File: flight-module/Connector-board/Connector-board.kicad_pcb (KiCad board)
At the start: 4 copper layers, 141.7 x 134.1 mm, 39 parts, among them J1 DB9_Female, J2 Stack_Shape, J3 DB9_Female, J4 DB15_Female, J5 DB25_Receptacle, U1 MAX31855KASA, U2 MAX31855KASA, U3 MAX31855KASA, U4 MAX31855KASA

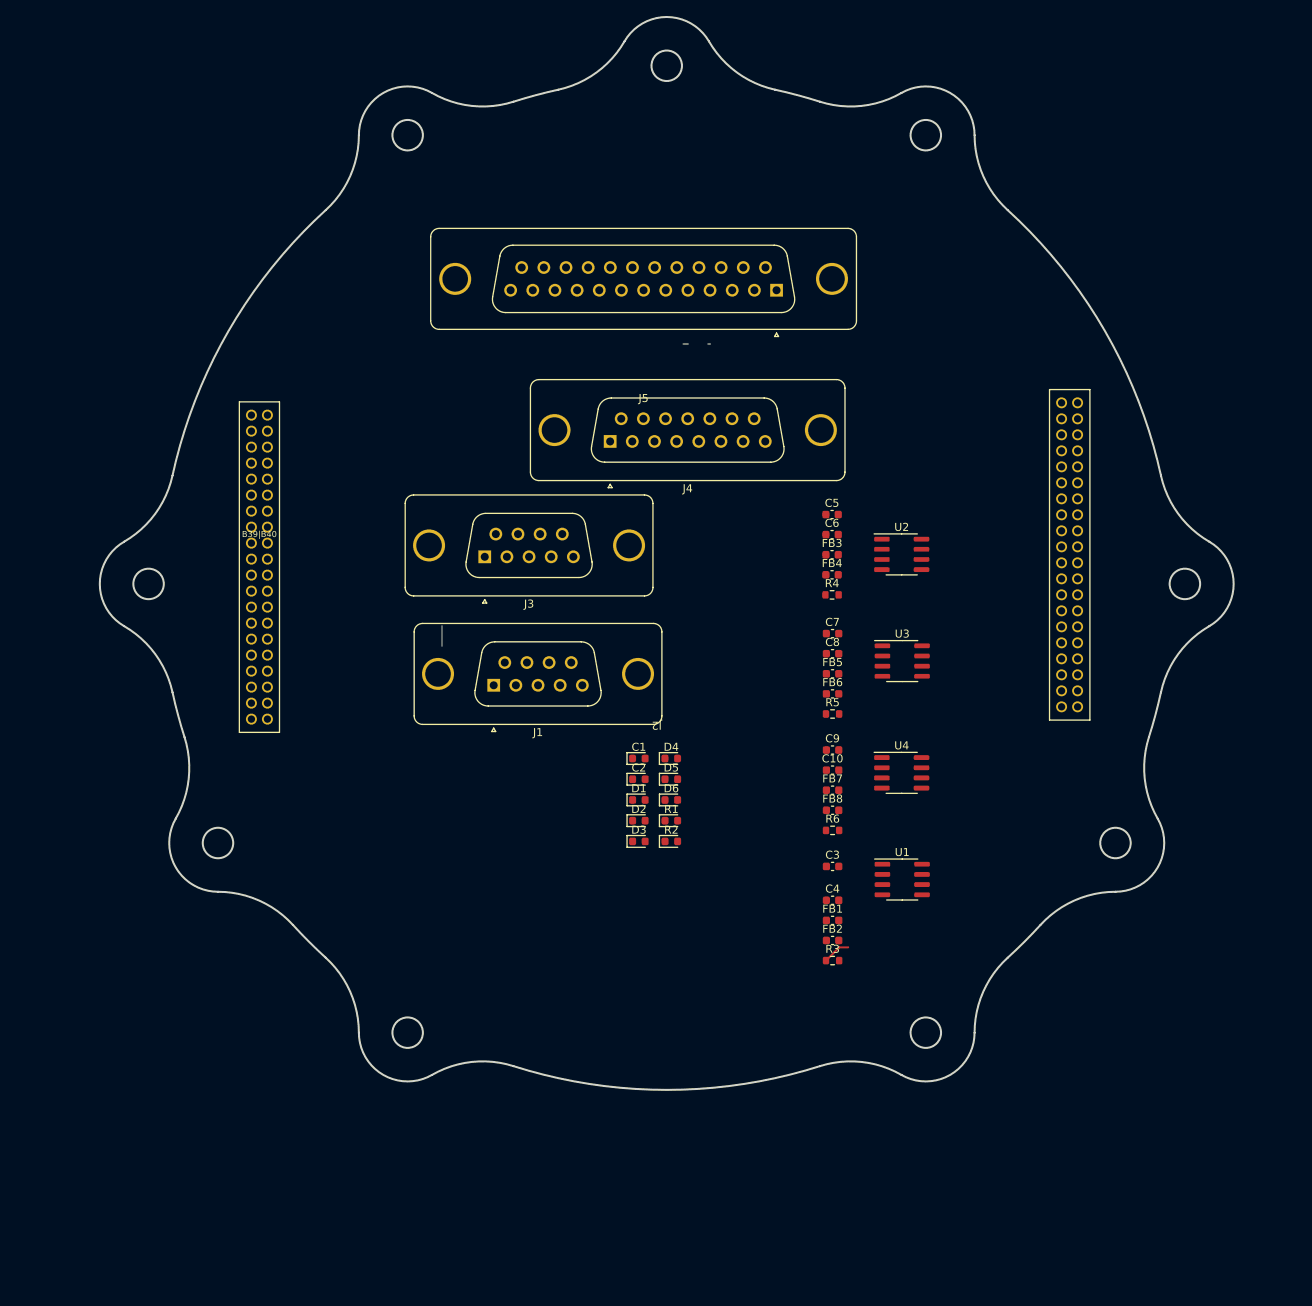
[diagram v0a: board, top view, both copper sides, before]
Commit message: completed routing
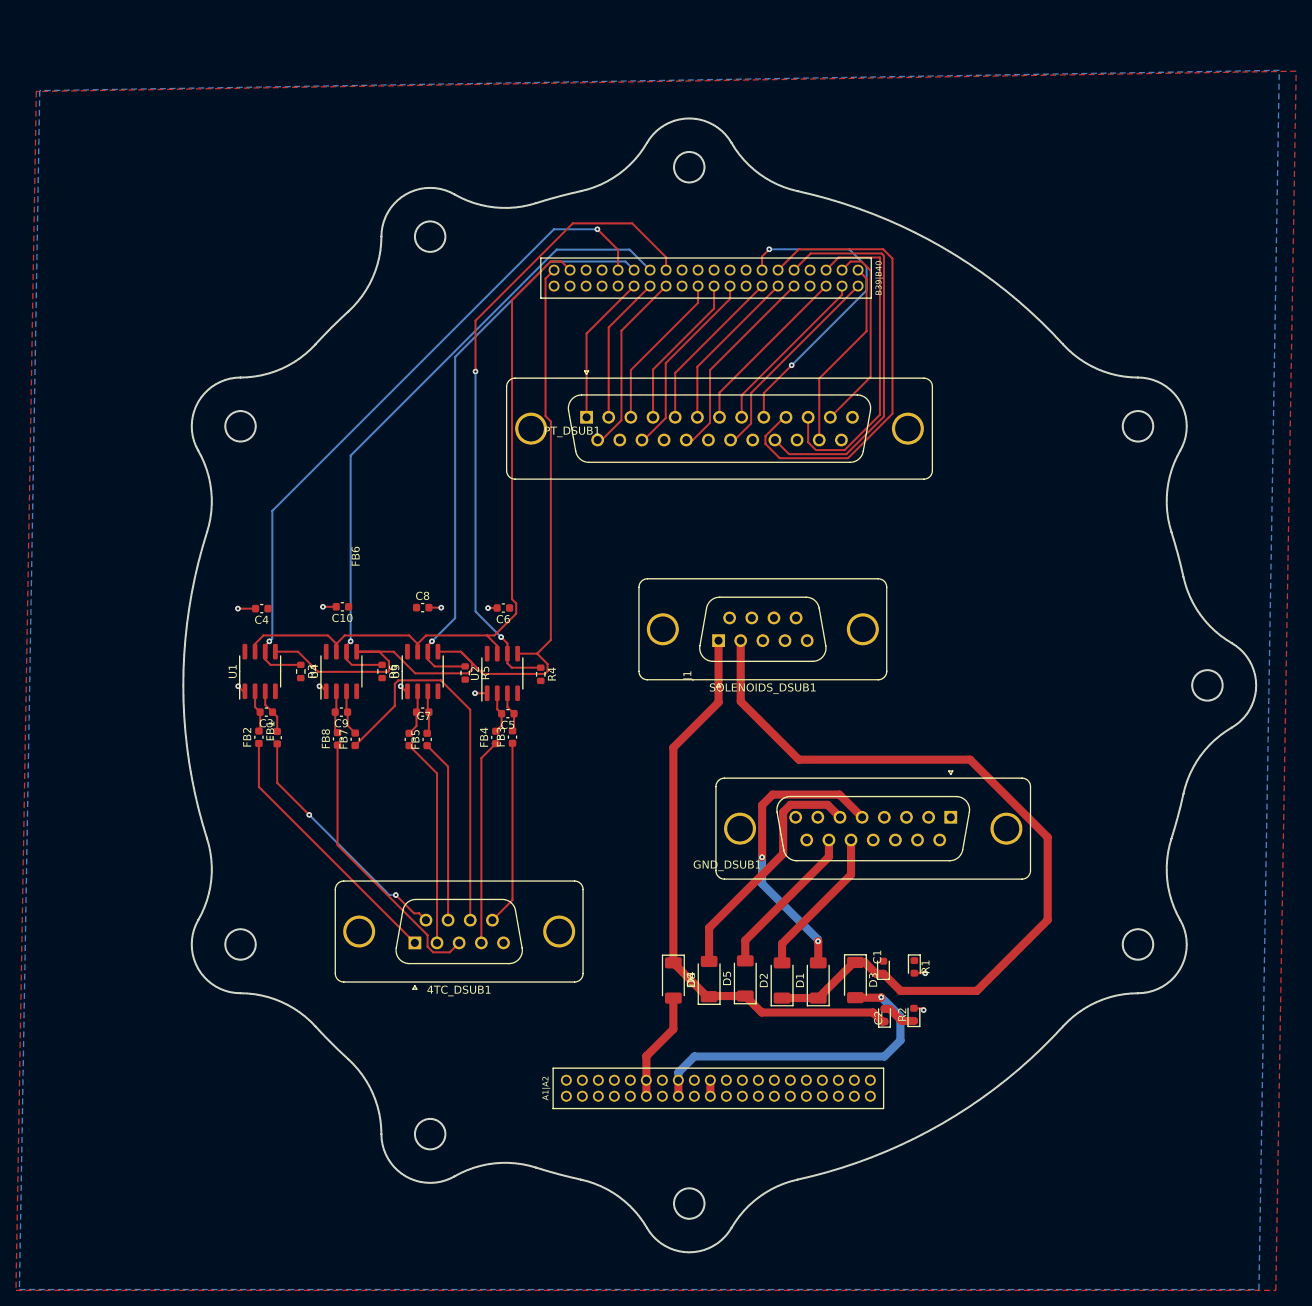
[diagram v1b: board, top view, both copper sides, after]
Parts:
- removed J2: Stack_Shape, Stack_Shape:Stack_Shape
- added J1: Stack_Shape, Stack_Shape:Stack_Shape, F.Cu at (172.7, 106.8)
- D1, D2, D3, D4, D5, D6: footprint Diode_SMD:D_0603_1608Metric -> Diode_SMD:D_SOD-128
- moved U1 84.4 mm to (117.9, 106.1), turned to 90 degrees
- moved C4 80.1 mm to (118.1, 98.2), turned to 180 degrees
- moved FB2 76.1 mm to (117.7, 114.3), turned to 90 degrees
- moved R3 75.7 mm to (122.9, 106.1), turned to -90 degrees
- moved C3 73.4 mm to (118.6, 111.2), turned to 180 degrees
- moved FB1 73.1 mm to (120.0, 114.3), turned to 90 degrees
- moved U4 71.2 mm to (128.0, 106.1), turned to 90 degrees
- moved C10 64.6 mm to (128.1, 98.0), turned to 180 degrees
- moved GND_DSUB1 63.4 mm to (204.2, 124.3), turned to 0 degrees
- moved FB8 62.5 mm to (127.5, 114.5), turned to 90 degrees
- moved C9 61.6 mm to (128.0, 111.2), turned to 180 degrees
- moved FB7 60.0 mm to (129.7, 114.6), turned to 90 degrees
- moved U3 60.0 mm to (138.2, 106.1), turned to 90 degrees
- moved R6 59.7 mm to (133.1, 106.1), turned to -90 degrees
- moved FB6 53.2 mm to (136.5, 114.6), turned to 90 degrees
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- renumbered J3 to 4TC_DSUB1, J4 to GND_DSUB1, J5 to PT_DSUB1, J1 to SOLENOIDS_DSUB1
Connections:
- C1 pad 1: /ETH_VENT -> ETH_VENT
- C2 pad 1: /LOX_VENT -> LOX_VENT
- D1 pad 1: /ETH_VENT -> ETH_VENT
- D2 pad 1: /ETH_VENT -> ETH_VENT
- D3 pad 1: /ETH_VENT -> ETH_VENT
- D4 pad 1: /LOX_VENT -> LOX_VENT
- D5 pad 1: /LOX_VENT -> LOX_VENT
- D6 pad 1: /LOX_VENT -> LOX_VENT
- GND_DSUB1 pad 14: GROUND_LOX_VENT -> REDS_LOX_VENT
- GND_DSUB1 pad 6: REDS_LOX_VENT -> GROUND_LOX_VENT
- PT_DSUB1 pad 10: unconnected-(J5-Pad10) -> PT5_E-
- PT_DSUB1 pad 11: unconnected-(J5-Pad11) -> PT6_E+
- PT_DSUB1 pad 12: unconnected-(J5-Pad12) -> PT6_E-
- PT_DSUB1 pad 15: PT2_E- -> unconnected-(PT_DSUB1-P15-Pad15)
- PT_DSUB1 pad 17: PT3_A+ -> unconnected-(PT_DSUB1-P17-Pad17)
- PT_DSUB1 pad 18: PT4_E- -> PT3_A+
- PT_DSUB1 pad 19: PT4_A+ -> unconnected-(PT_DSUB1-P19-Pad19)
- PT_DSUB1 pad 20: PT5_A+ -> PT4_A+
- PT_DSUB1 pad 21: PT6_E+ -> unconnected-(PT_DSUB1-P21-Pad21)
- PT_DSUB1 pad 22: PT6_E- -> PT5_A+
- PT_DSUB1 pad 24: unconnected-(J5-P24-Pad24) -> PT6_A+
- PT_DSUB1 pad 4: PT3_E+ -> PT2_E-
- PT_DSUB1 pad 5: PT3_E- -> PT3_E+
- PT_DSUB1 pad 6: PT4_E+ -> PT3_E-
- PT_DSUB1 pad 7: PT5_E+ -> PT4_E+
- PT_DSUB1 pad 8: PT5_E- -> PT4_E-
- PT_DSUB1 pad 9: PT6_A+ -> PT5_E+
- SOLENOIDS_DSUB1 pad 1: LOX_VENT+ -> LOX_VENT
- SOLENOIDS_DSUB1 pad 2: ETH_VENT+ -> ETH_VENT
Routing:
- net SPI_SCK: track 0.00 -> 110.3 mm
- net ETH_VENT: track 0.00 -> 104.0 mm
- net SPI_MISO: track 0.00 -> 92.2 mm
- net TC1_CS: track 3.46 -> 85.4 mm, vias 0 -> 2
- net TC4_CS: track 0.00 -> 81.2 mm, vias 0 -> 2
- net TC3_CS: track 0.00 -> 79.9 mm, vias 0 -> 1
- net TC2_CS: track 0.00 -> 72.6 mm, vias 0 -> 1
- net LOX_VENT: track 0.00 -> 72.4 mm
- net PT5_E-: track 0.00 -> 58.7 mm
- net PT5_A+: track 0.00 -> 48.6 mm
- net TC3_T+: track 0.00 -> 47.2 mm
- net FLIGHT_ETH_VENT: track 0.00 -> 42.0 mm, vias 0 -> 1
- net PT6_E+: track 0.00 -> 41.4 mm
- net PT5_E+: track 0.00 -> 40.2 mm, vias 0 -> 2
- net GROUND_ETH_VENT: track 0.00 -> 36.5 mm, vias 0 -> 2
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- added copper zone on F.Cu, net +3.3V
- added copper zone on B.Cu, net +5V
- added copper zone on In2.Cu, net PWR_SUP
- removed copper zone on In2.Cu, net +3.3V
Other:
- board size 141.7 x 134.1 mm -> 134.1 x 141.7 mm
